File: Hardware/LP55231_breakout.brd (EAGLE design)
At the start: 25.4 x 25.4 mm, 13 parts

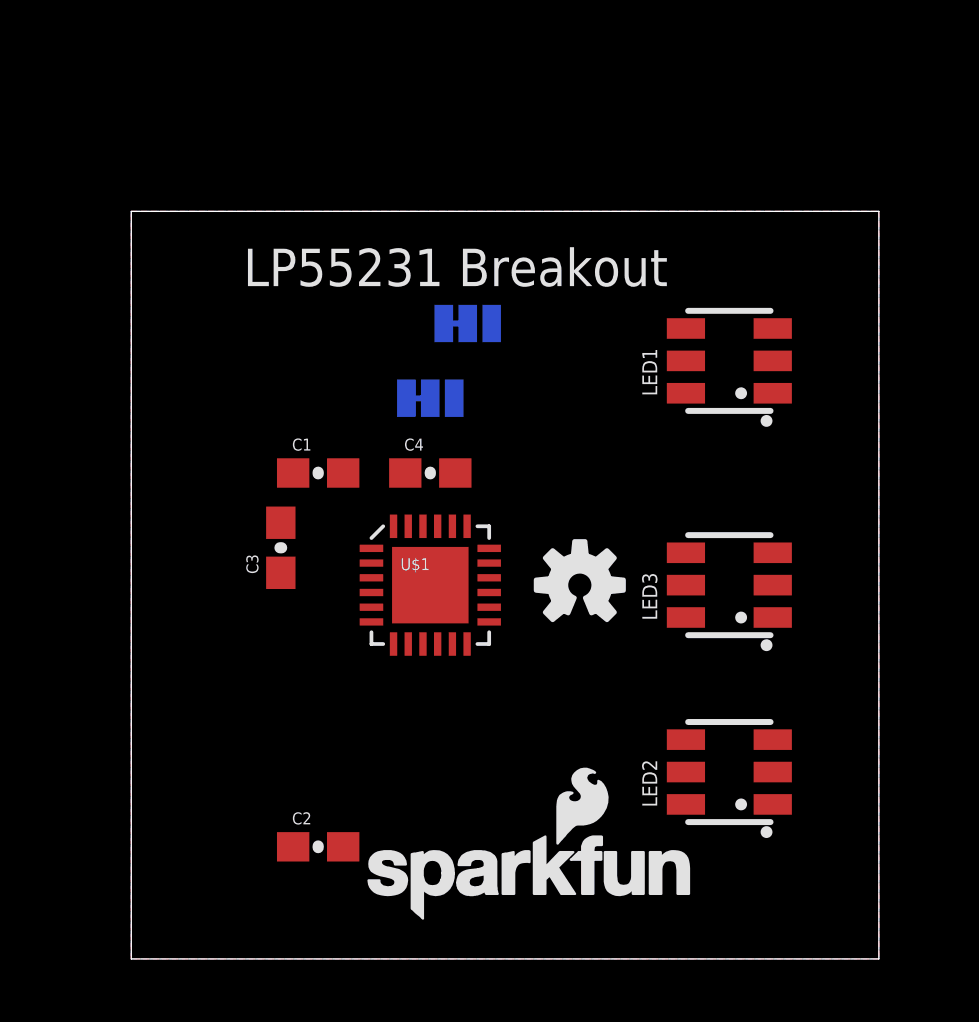
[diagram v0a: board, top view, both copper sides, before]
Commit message: PCB Work in progress.
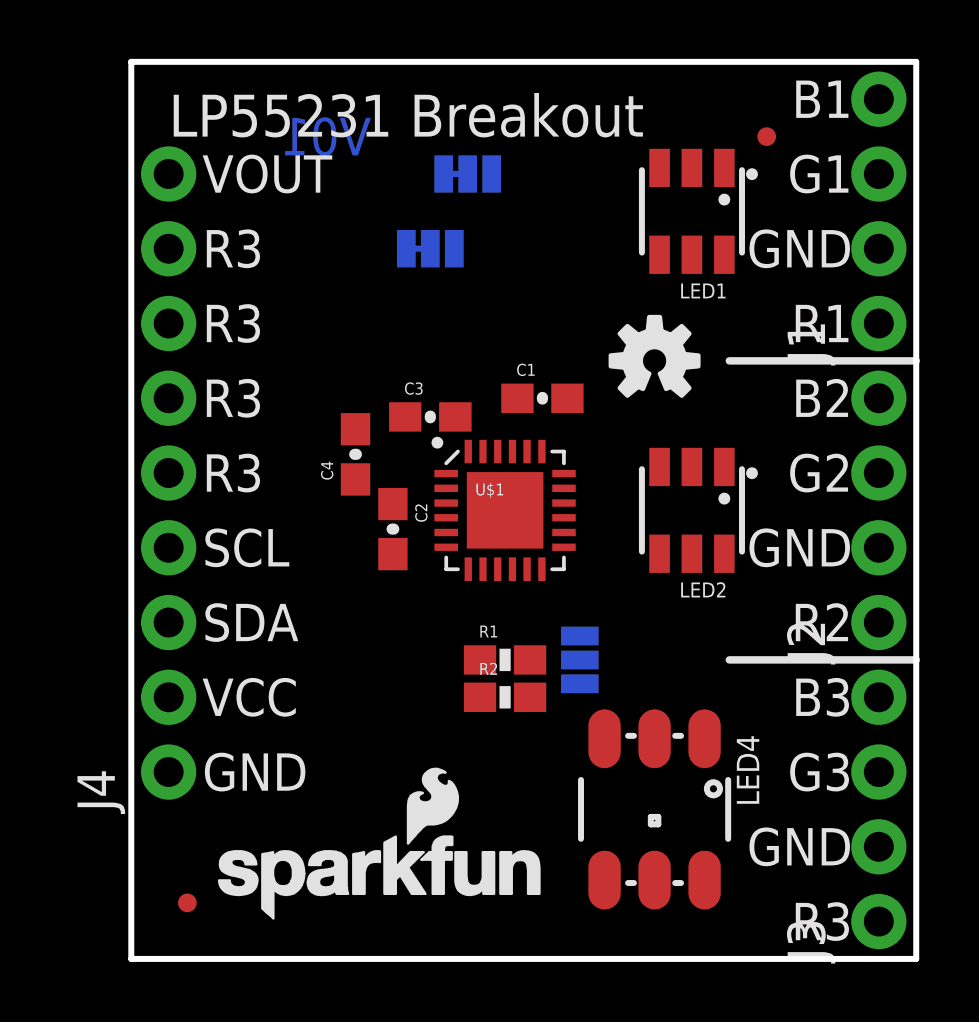
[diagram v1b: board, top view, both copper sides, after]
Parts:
- removed LED3: LED-TRICOLOR-NO-COMPLCC-6-SMD, SparkFun-LED:PLCC-6-LED
- added FD1, FD2: FIDUCIALUFIDUCIAL, SparkFun-Aesthetics:MICRO-FIDUCIAL
- added J1, J2, J3: (no value), SparkFun-Connectors:1X04_NO_SILK_ALL_ROUND
- added J4: (no value), SparkFun-Connectors:1X09_NO_SILK
- added JP3: I2C-PULLUPS, SparkFun-Passives:PAD-JUMPER-3-NC_BY_PASTE_YES_SILK_FULL_BOX
- added LED4: LED-TRICOLOR-5050NO_IC, SparkFun-LED:LED-TRICOLOR-5050
- added R1, R2: 4.7K, SparkFun-Resistors:0603-RES
- moved C2 11.1 mm to (8.89, 14.6), turned to 270 degrees
- moved LED2 8.98 mm to (19.1, 15.2), turned to 180 degrees
- moved LOGO1 8.03 mm to (17.8, 20.3)
- moved C1 8.03 mm to (14.0, 19.1)
- moved C3 6.75 mm to (10.2, 18.4), turned to 0 degrees
- moved LED1 5.24 mm to (19.1, 25.4), turned to 180 degrees
- moved JP1 5.08 mm to (11.4, 26.7)
- moved LOGO2 5.08 mm to (2.54, 1.27)
- moved JP2 5.08 mm to (10.2, 24.1)
- moved U$1 3.59 mm to (12.7, 15.2)
- moved C4 2.62 mm to (7.62, 17.1), turned to 90 degrees
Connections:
- net N$16 renamed ADDR1
- net N$17 renamed ADDR0
- removed net N$1: LED3.AR, U$1.11
- removed net N$10: C1.1, U$1.22
- removed net N$2: LED3.AG, U$1.15
- removed net N$3: LED3.AB, U$1.14
- removed net N$4: LED2.AB, U$1.16
- removed net N$5: LED2.AR, U$1.12
- removed net N$6: LED2.AG, U$1.17
- removed net N$7: LED1.AR, U$1.13
- removed net N$8: LED1.AG, U$1.19
- removed net N$9: LED1.AB, U$1.18
- new net B1: J1.4, LED1.AB, U$1.18
- new net B2: J2.4, LED2.AB, U$1.16
- new net B3: J3.4, LED4.3, U$1.14
- new net G1: J1.3, LED1.AG, U$1.19
- new net G2: J2.3, LED2.AG, U$1.17
- new net G3: J3.3, LED4.1, U$1.15
- new net N$15: U$1.7
- new net N$18: U$1.10
- new net N$19: U$1.5
- new net N$20: U$1.6
- new net N$21: JP3.1, R2.2
- new net N$22: JP3.3, R1.2
- new net R1: J1.1, LED1.AR, U$1.13
- new net R2: J2.1, LED2.AR, U$1.12
- new net R3: J3.1, LED4.2, U$1.11
- new net SCL: J4.4, R1.1, U$1.9
- new net SDA: J4.3, R2.1, U$1.8
- new net VOUT: C1.1, J4.9, U$1.22
- net GND: now also J1.2, J2.2, J3.2, J4.1, LED4.4, LED4.5, LED4.6; no longer LED3.CB, LED3.CG, LED3.CR
- net VCC: now also J4.2, JP3.2
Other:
- board size 25.4 x 25.4 mm -> 26.7 x 30.5 mm
- board text added: "B1"
- board text added: "B2"
- board text added: "B3"
- board text added: "G1"
- board text added: "G2"
- board text added: "G3"
- board text added: "GND"
- board text added: "R1"
- board text added: "R2"
- board text added: "R3"
- board text added: "SCL"
- board text added: "SDA"
- board text added: "V01"
- board text added: "VCC"
- board text added: "VOUT"
